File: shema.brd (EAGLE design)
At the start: 100 x 80 mm, 20 parts

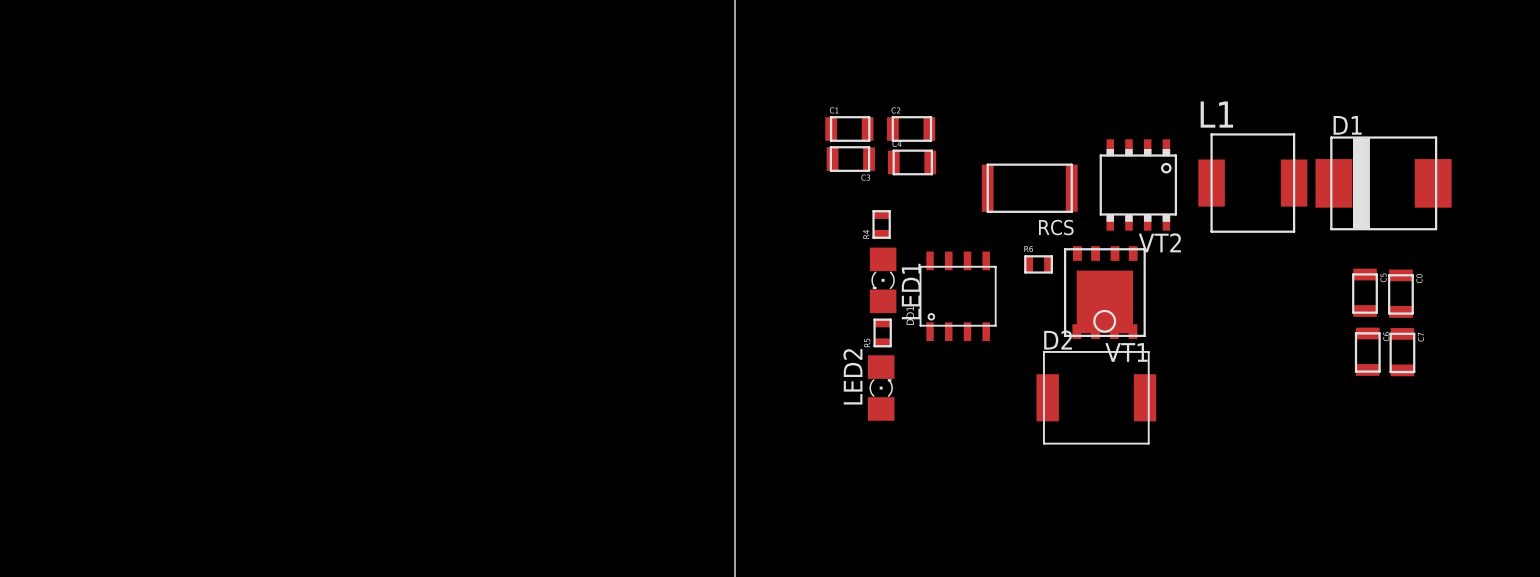
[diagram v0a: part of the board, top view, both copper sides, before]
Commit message: изменения файлов
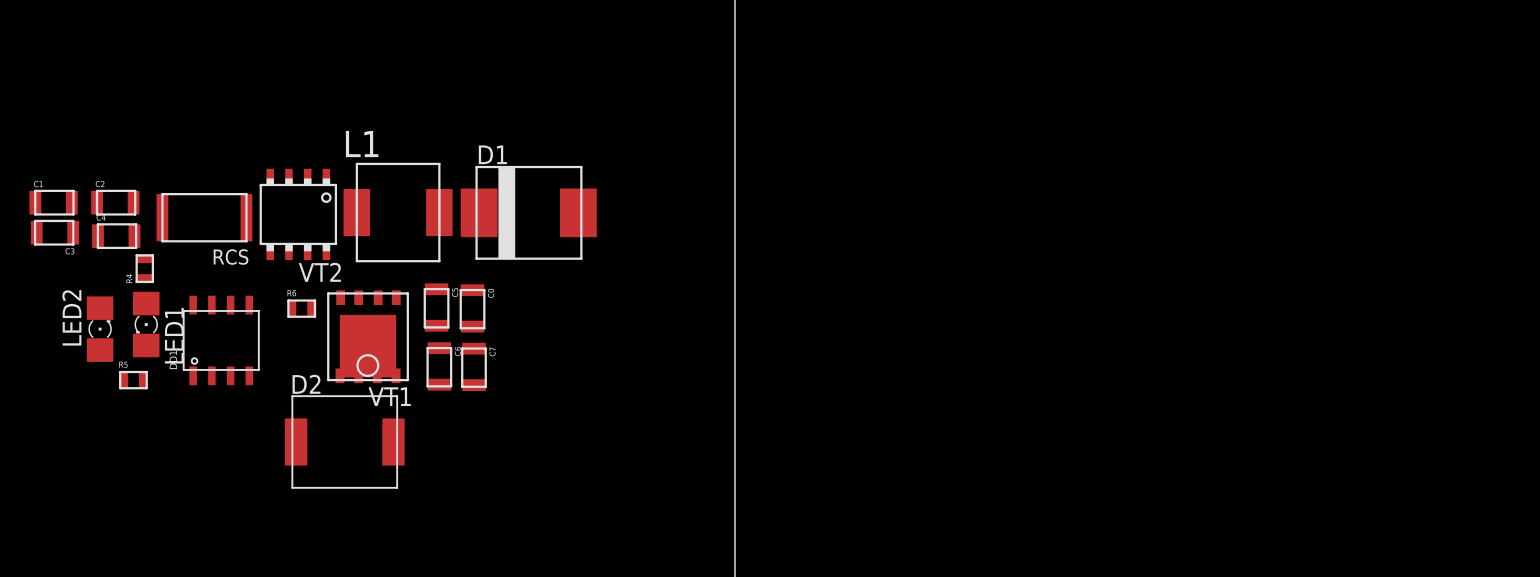
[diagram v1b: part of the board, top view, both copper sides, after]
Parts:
- moved C0 63.0 mm to (-17.8, 24.9)
- moved C5 63.0 mm to (-20.2, 24.9)
- moved C6 63.0 mm to (-20.1, 20.9)
- moved C7 63.0 mm to (-17.7, 20.9)
- moved D1 58.0 mm to (-14.0, 31.3)
- moved L1 58.0 mm to (-22.9, 31.4)
- moved VT2 57.0 mm to (-29.6, 31.2)
- moved RCS 56.0 mm to (-36.0, 31.0)
- moved C1 54.2 mm to (-46.2, 32.0)
- moved C2 54.2 mm to (-42.0, 32.0)
- moved C3 54.2 mm to (-46.1, 30.0)
- moved C4 54.2 mm to (-42.0, 29.8)
- moved LED2 53.2 mm to (-43.1, 23.4)
- moved D2 51.1 mm to (-26.5, 15.8)
- moved R5 50.9 mm to (-40.8, 20.0), turned to 0 degrees
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
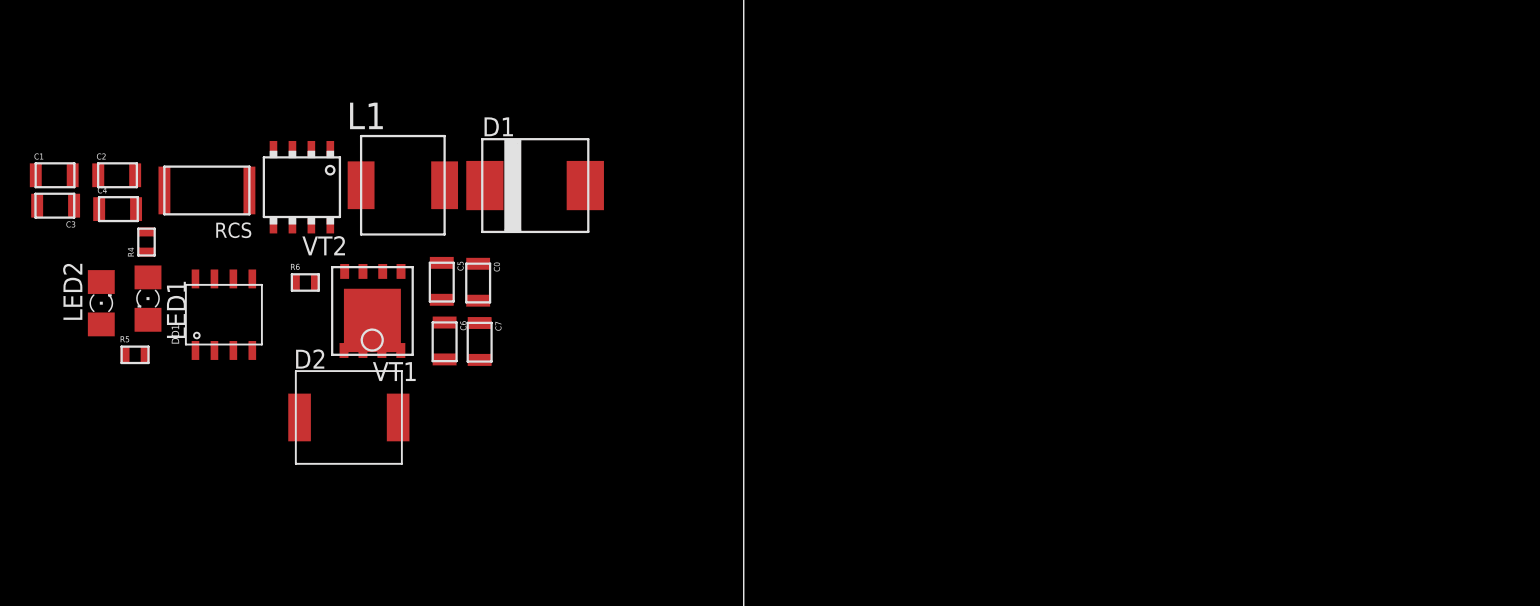
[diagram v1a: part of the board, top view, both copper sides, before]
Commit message: изменение файлов
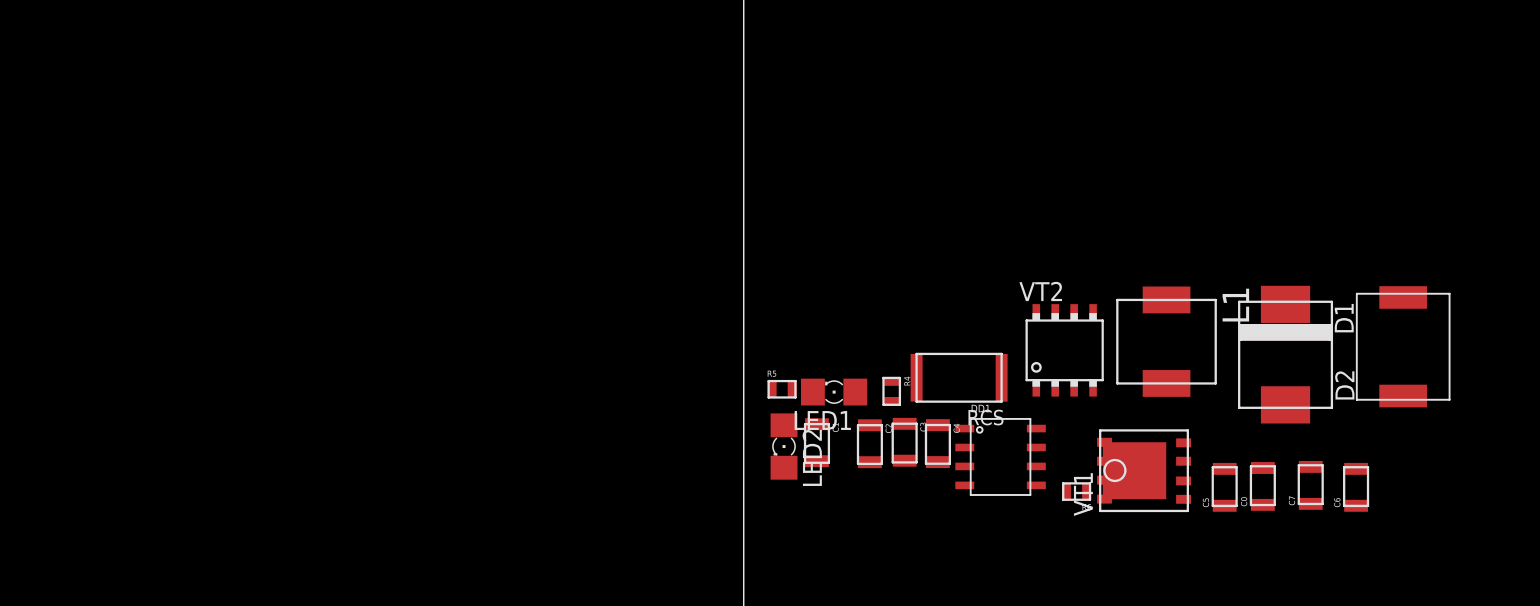
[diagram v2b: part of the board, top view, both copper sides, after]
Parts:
- moved D2 70.9 mm to (44.2, 20.5), turned to 90 degrees
- moved C6 61.9 mm to (41.1, 11.1), turned to 90 degrees
- moved C3 59.1 mm to (10.8, 14.1), turned to 270 degrees
- moved C4 57.2 mm to (13.0, 14.0), turned to 270 degrees
- moved C7 56.6 mm to (38.0, 11.2), turned to 90 degrees
- moved C0 54.4 mm to (34.8, 11.2), turned to 90 degrees
- moved C5 54.3 mm to (32.2, 11.1), turned to 90 degrees
- moved C1 54.2 mm to (4.91, 14.1), turned to 270 degrees
- moved C2 53.6 mm to (8.46, 14.0), turned to 270 degrees
- moved R6 53.6 mm to (22.3, 10.8), turned to 180 degrees
- moved DD1 52.9 mm to (17.2, 13.1), turned to 270 degrees
- moved VT1 52.8 mm to (26.8, 12.2), turned to 90 degrees
- moved VT2 52.3 mm to (21.5, 20.3), turned to 0 degrees
- moved L1 52.3 mm to (28.4, 20.9), turned to 270 degrees
- moved RCS 52.0 mm to (14.4, 18.4)
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
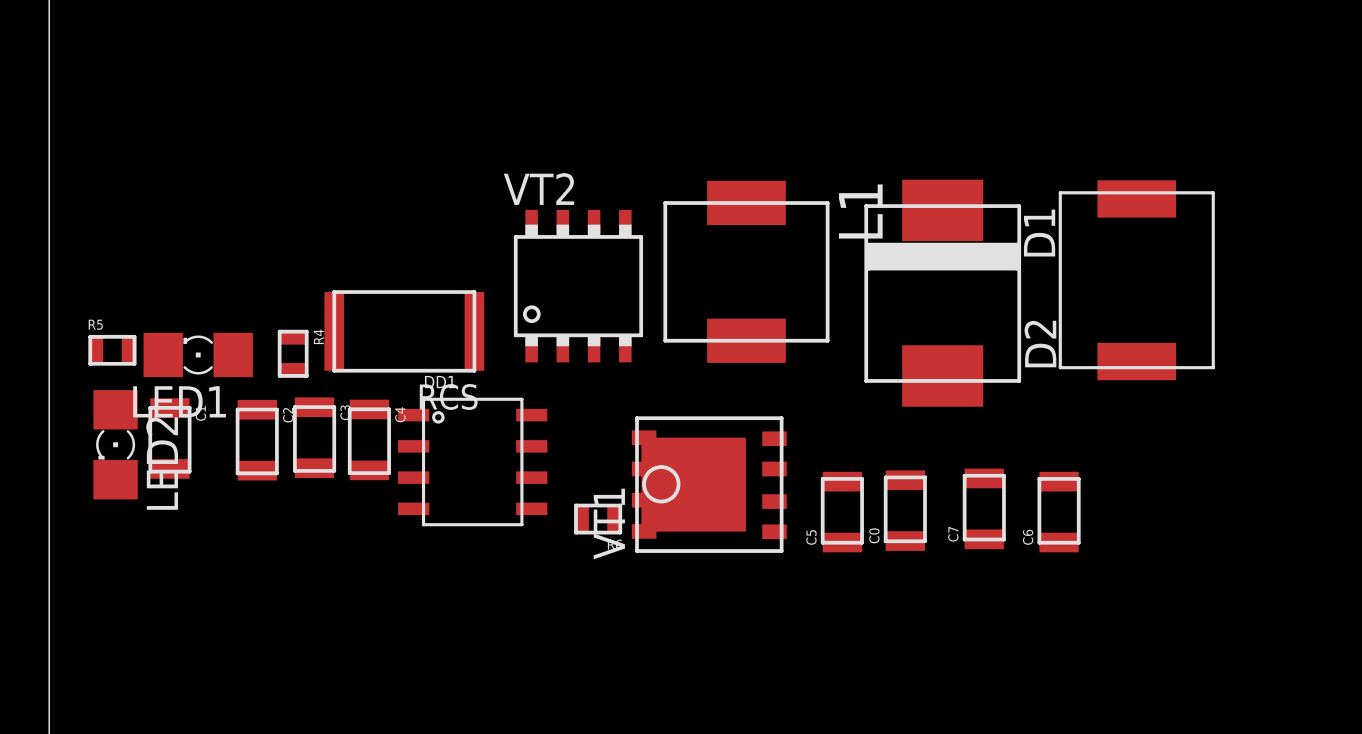
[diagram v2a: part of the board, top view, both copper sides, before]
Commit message: изменение файлов
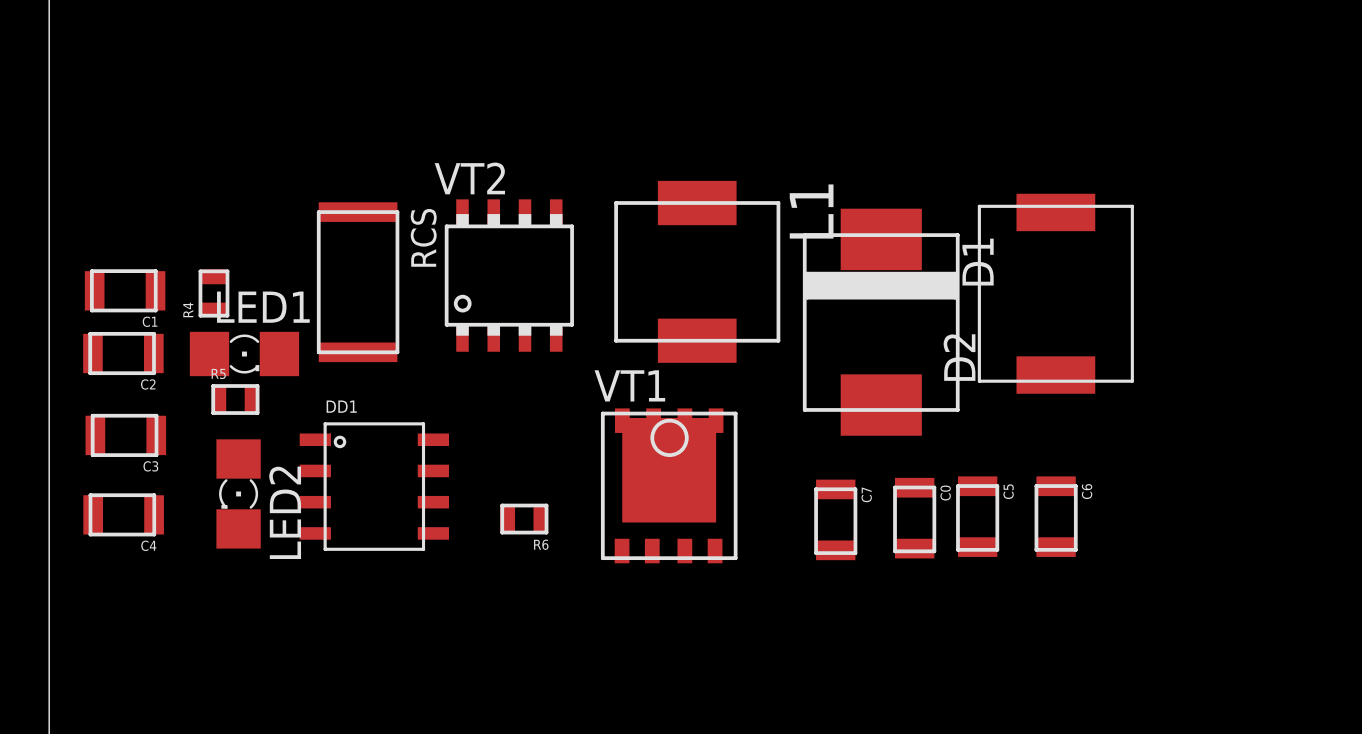
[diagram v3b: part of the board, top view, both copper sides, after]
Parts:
- moved C4 10.4 mm to (3.03, 11.0), turned to 180 degrees
- moved C3 7.67 mm to (3.12, 14.2), turned to 180 degrees
- moved C2 6.48 mm to (3.02, 17.5), turned to 180 degrees
- moved C1 6.27 mm to (3.09, 20.1), turned to 180 degrees
- moved C7 6.06 mm to (32.0, 10.8), turned to 270 degrees
- moved C5 5.50 mm to (37.8, 10.9), turned to 270 degrees
- moved LED2 5.39 mm to (7.70, 11.8)
- moved R5 5.39 mm to (7.57, 15.7)
- moved DD1 4.12 mm to (13.2, 12.1)
- moved R4 4.05 mm to (6.70, 20.0), turned to 90 degrees
- moved D2 3.34 mm to (40.9, 20.0)
- moved R6 3.00 mm to (19.3, 10.8)
- moved VT2 2.84 mm to (18.7, 20.7)
- moved D1 2.76 mm to (33.8, 18.8)
- moved RCS 2.74 mm to (12.6, 20.4), turned to 270 degrees
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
